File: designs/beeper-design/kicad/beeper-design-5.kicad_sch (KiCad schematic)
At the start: 1 part, among them U5 FH19C-6S-0.5SH(10)

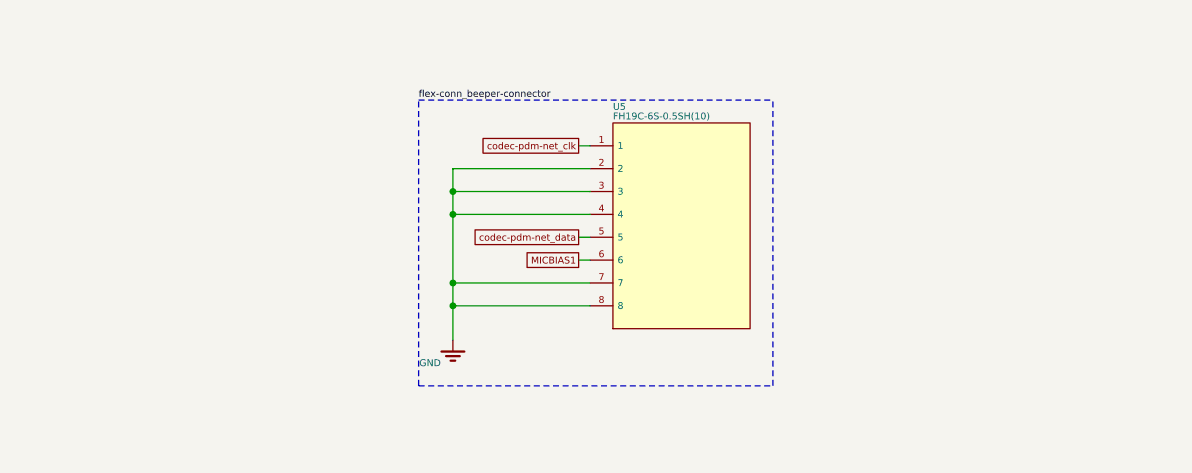
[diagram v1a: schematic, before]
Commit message: another export
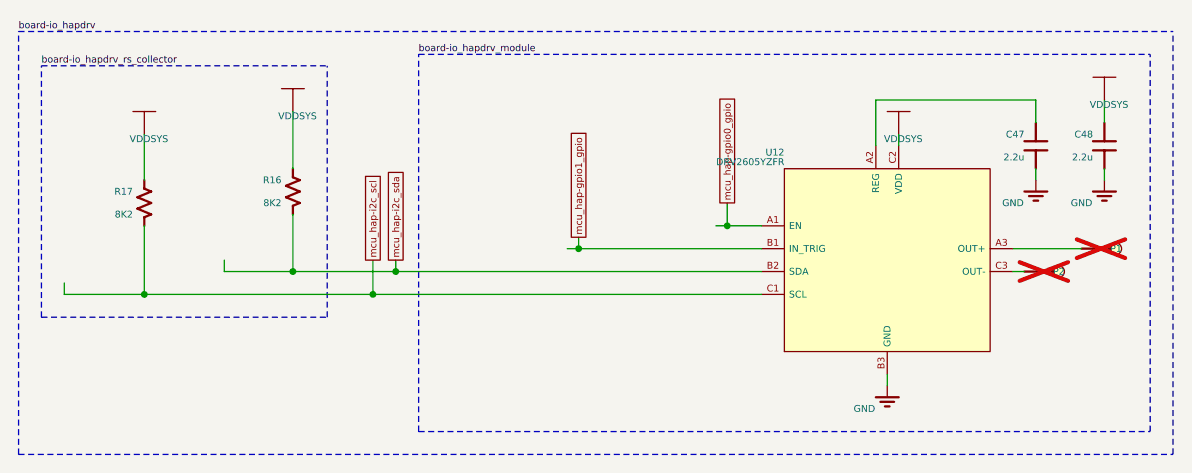
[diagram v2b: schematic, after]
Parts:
- removed U5: FH19C-6S-0.5SH(10), beeper-design:LP_4, symbol FH19C_6S_0_5SH_10_
- added C47: 2.2u, beeper-design:Pkg0201_11, symbol C335106_9
- added C48: 2.2u, beeper-design:Pkg0201_24, symbol C335106_17
- added R16, R17: 8K2, beeper-design:Pkg0201_39, symbol my_resistor_9
- added TP1, TP2: (no value), beeper-design:SMD_TESTPT, symbol smd_testpoint_cmp
- added U12: DRV2605YZFR, beeper-design:LP_7, symbol DRV2605YZFR
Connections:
- net GND: now also C47.1, C48.1, U12.B3 (GND)
- new net: C47.2, U12.A2 (REG)
- new net: TP1.p, U12.A3 (OUT+)
- new net: TP2.p, U12.C3 (OUT-)
- new net VDDSYS: C48.2, R16.2, R17.2, U12.C2 (VDD)
- new net mcu_hap-gpio0_gpio: U12.A1 (EN)
- new net mcu_hap-gpio1_gpio: U12.B1 (IN_TRIG)
- new net mcu_hap-i2c_scl: R17.1, U12.C1 (SCL)
- new net mcu_hap-i2c_sda: R16.1, U12.B2 (SDA)
